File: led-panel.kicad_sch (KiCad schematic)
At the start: 0 parts

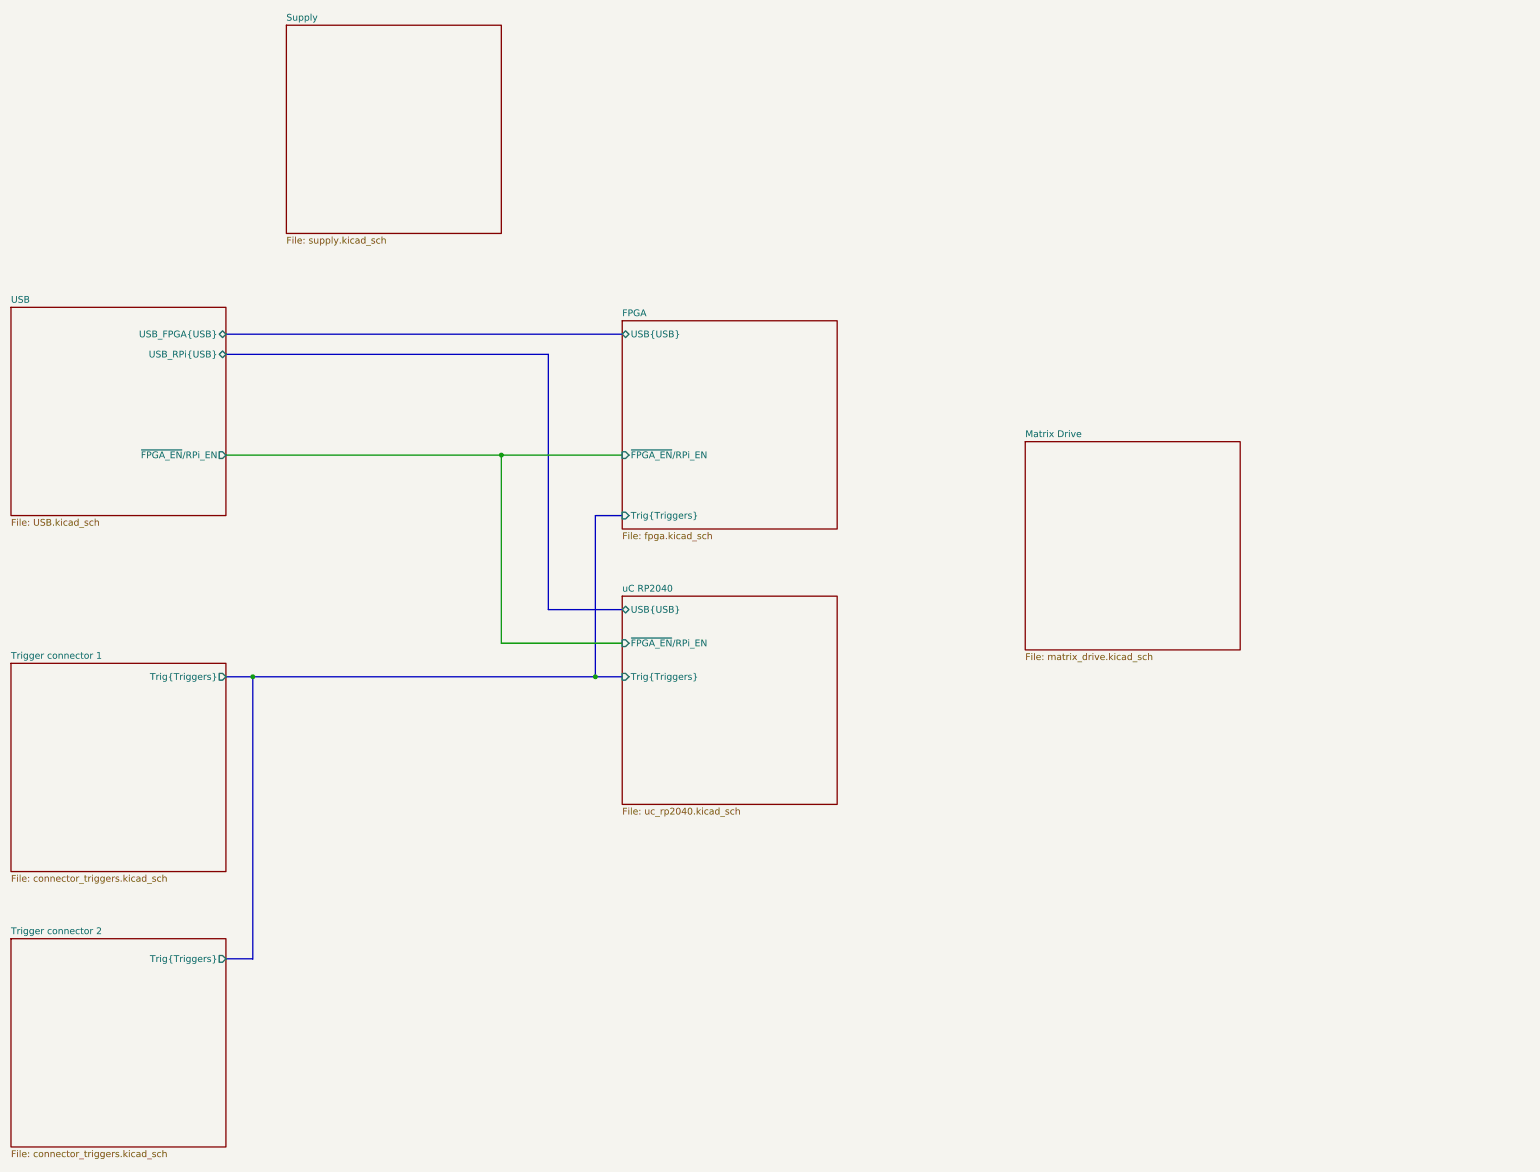
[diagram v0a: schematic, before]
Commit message: [#72133] Add LED matrix
Signed-off-by: Dawid Lentka <dlentka@antmicro.com>
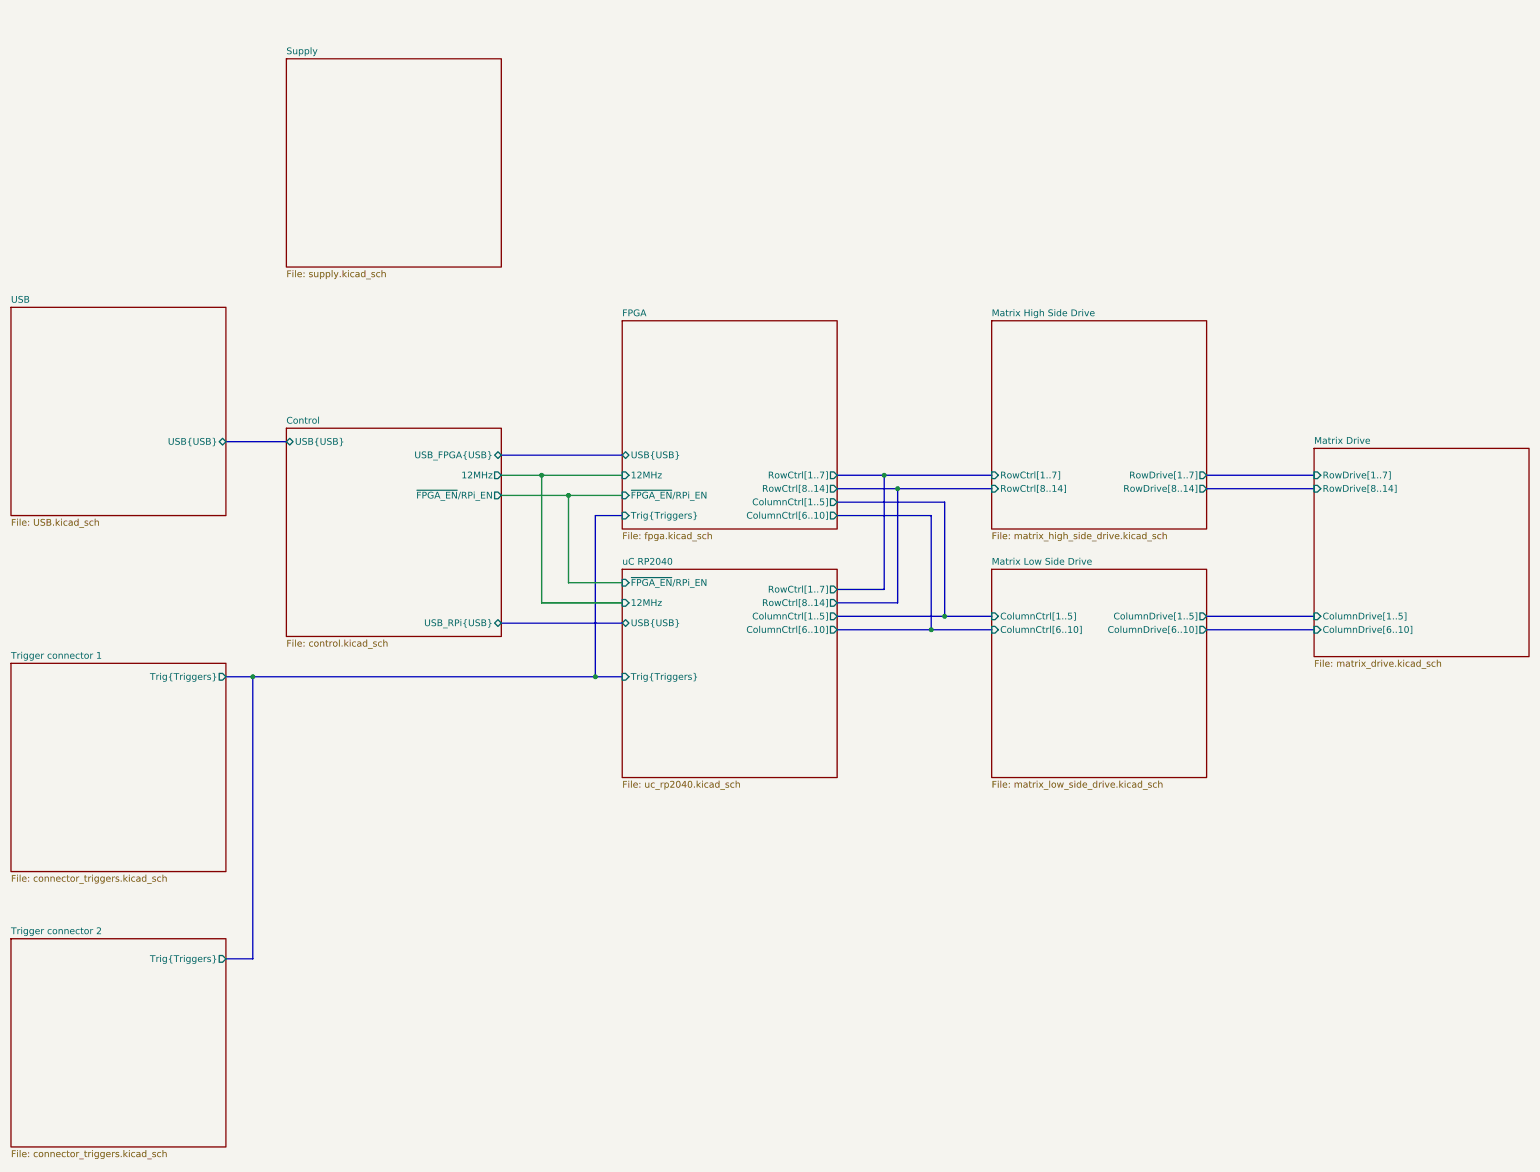
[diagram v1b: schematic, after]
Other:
- added sheet Control (control.kicad_sch)
- added sheet Matrix High Side Drive (matrix_high_side_drive.kicad_sch)
- added sheet Matrix Low Side Drive (matrix_low_side_drive.kicad_sch)
- sheet FPGA ports: added 12MHz, ColumnCtrl[1..5], ColumnCtrl[6..10], RowCtrl[1..7], RowCtrl[8..14]; removed none
- sheet Matrix Drive ports: added ColumnDrive[1..5], ColumnDrive[6..10], RowDrive[1..7], RowDrive[8..14]; removed none
- sheet USB ports: added USB{USB}; removed USB_FPGA{USB}, USB_RPi{USB}, ~{FPGA_EN}/RPi_EN
- sheet uC RP2040 ports: added 12MHz, ColumnCtrl[1..5], ColumnCtrl[6..10], RowCtrl[1..7], RowCtrl[8..14]; removed none
